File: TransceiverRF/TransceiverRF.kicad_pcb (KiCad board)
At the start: 2 copper layers, 48 parts, among them U1 CC1101, U2 CON_SMA, U3 CC2500, U4 CON_SMA, Y1 26 MHz, Y2 26 MHz

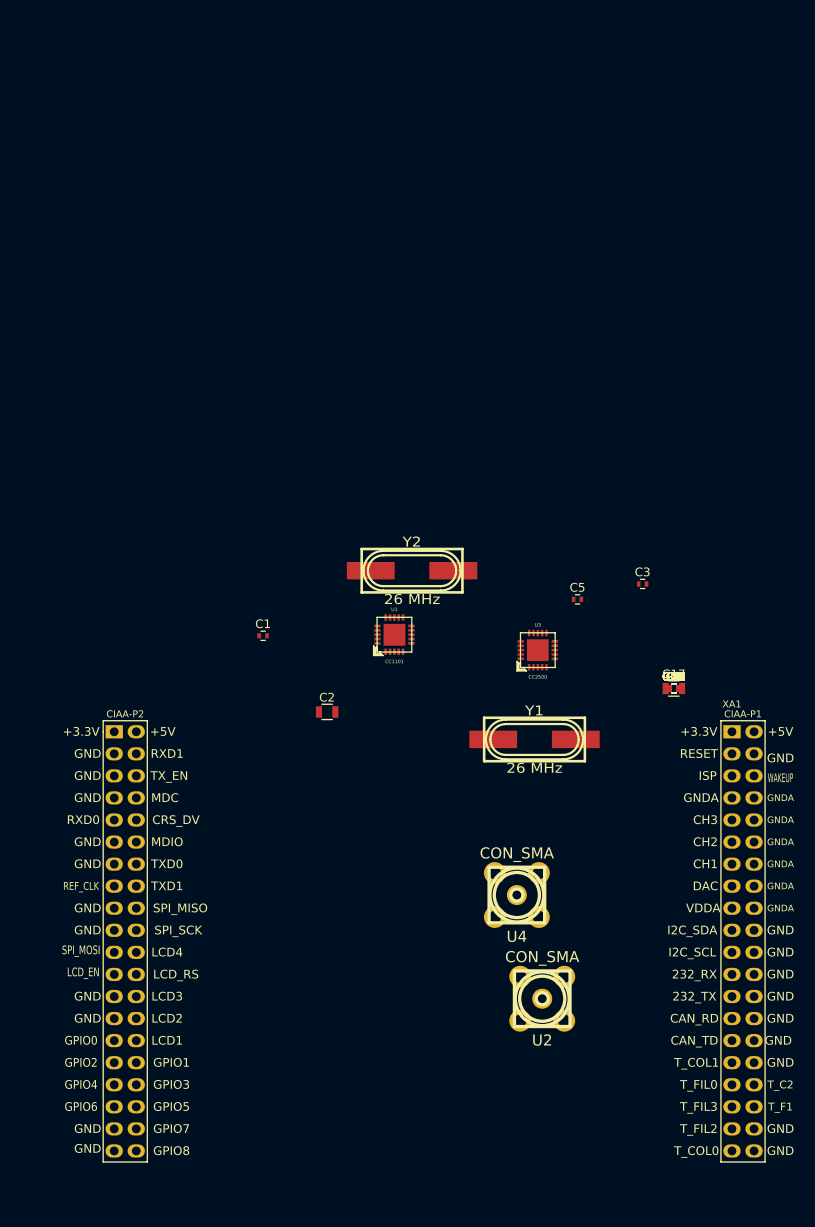
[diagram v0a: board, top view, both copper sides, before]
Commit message: agrego pcb
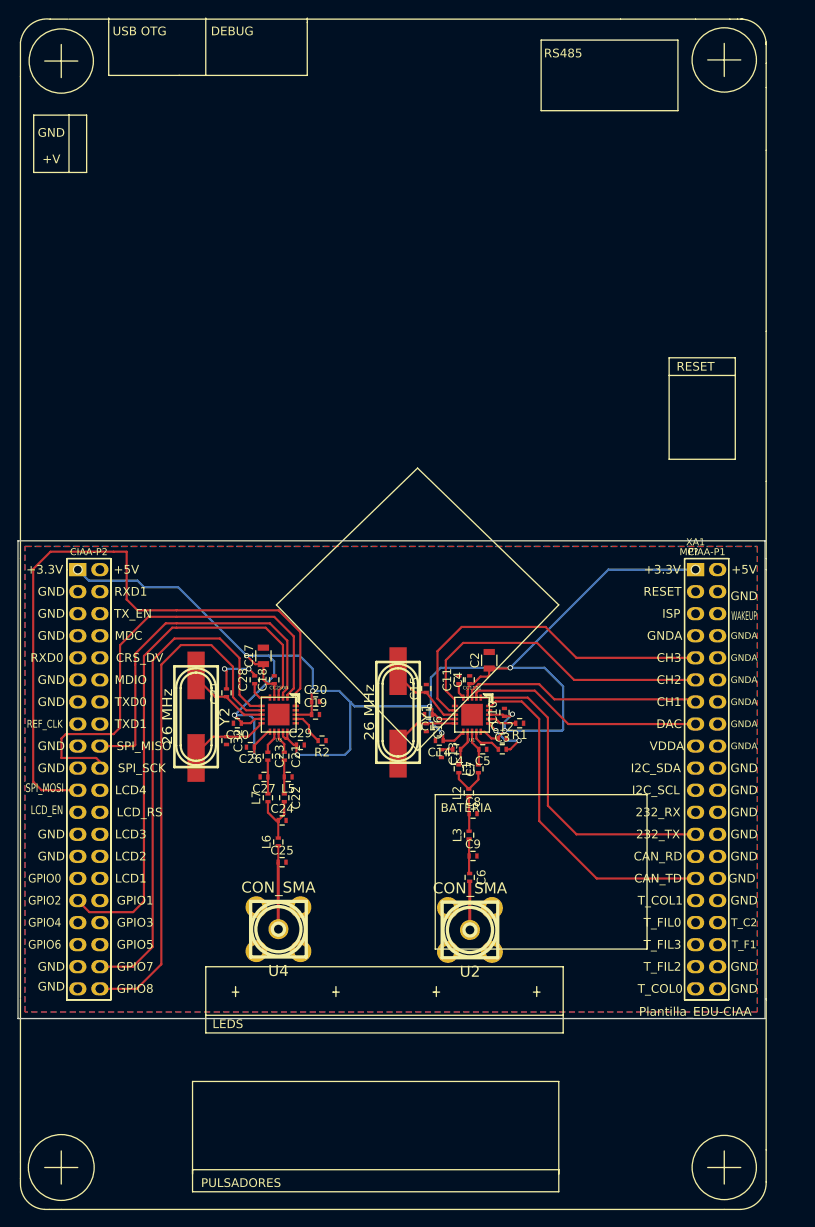
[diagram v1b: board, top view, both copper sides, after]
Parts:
- added MP?: Plantilla_EDU-CIAA, TransceiverRF:Plantilla_EDU-CIAA, F.Cu at (151.0, 91.3)
- moved C32 51.8 mm to (97.0, 111.0), turned to 270 degrees
- moved C31 51.5 mm to (97.0, 105.5), turned to 90 degrees
- moved C30 50.4 mm to (98.2, 109.0), turned to 180 degrees
- moved C25 49.3 mm to (103.4, 125.0)
- moved C26 49.2 mm to (99.8, 111.8), turned to 180 degrees
- moved L6 48.8 mm to (103.0, 122.7), turned to 90 degrees
- moved L7 48.4 mm to (101.8, 117.6), turned to 90 degrees
- moved C27 48.3 mm to (101.3, 115.2), turned to 180 degrees
- moved C28 48.3 mm to (100.2, 104.0), turned to 90 degrees
- moved C24 47.6 mm to (103.4, 120.2)
- moved C17 47.4 mm to (101.2, 101.2), turned to 90 degrees
- moved C23 47.4 mm to (101.8, 112.8), turned to 270 degrees
- moved C22 46.6 mm to (103.7, 117.6), turned to 270 degrees
- moved C18 46.0 mm to (102.5, 104.0), turned to 90 degrees
- moved L5 45.6 mm to (104.1, 115.2), turned to 180 degrees
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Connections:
- C1 pad 2: Net-(C1-Pad2) -> Earth
- C10 pad 2: Net-(C10-Pad2) -> Earth
- C11 pad 2: Net-(C11-Pad2) -> Earth
- C12 pad 2: Net-(C12-Pad2) -> Earth
- C13 pad 2: Net-(C13-Pad2) -> Earth
- C14 pad 2: Net-(C14-Pad2) -> Earth
- C15 pad 2: Net-(C15-Pad2) -> Earth
- C16 pad 2: Net-(C16-Pad2) -> Earth
- C17 pad 2: Net-(C17-Pad2) -> Earth
- C18 pad 2: Net-(C18-Pad2) -> Earth
- C19 pad 2: Net-(C19-Pad2) -> Earth
- C2 pad 2: Net-(C2-Pad2) -> Earth
- C20 pad 2: Net-(C20-Pad2) -> Earth
- C24 pad 2: Net-(C24-Pad2) -> Earth
- C25 pad 2: Net-(C25-Pad2) -> Earth
- C26 pad 2: Net-(C26-Pad2) -> Earth
- C27 pad 2: Net-(C27-Pad2) -> Earth
- C28 pad 2: Net-(C28-Pad2) -> Earth
- C29 pad 2: Net-(C29-Pad2) -> Earth
- C3 pad 2: Net-(C3-Pad2) -> Earth
- C30 pad 2: Net-(C30-Pad2) -> Earth
- C31 pad 2: Net-(C31-Pad2) -> Earth
- C32 pad 2: Net-(C32-Pad2) -> Earth
- C4 pad 2: Net-(C4-Pad2) -> Earth
- C5 pad 1: Net-(C5-Pad1) -> Earth
- C8 pad 2: Net-(C8-Pad2) -> Earth
- C9 pad 2: Net-(C9-Pad2) -> Earth
- L5 pad 1: Net-(L5-Pad1) -> Earth
- R1 pad 1: Net-(R1-Pad1) -> Earth
- R2 pad 1: Net-(R2-Pad1) -> Earth
- U1 pad 16: Net-(U1-Pad16) -> Earth
- U1 pad 19: Net-(U1-Pad19) -> Earth
- U1 pad 3: /Conectores/GDO1(opcional)_CC1101 -> /CC1101/GDO2(opcional)_CC1101
- U2 pad 2: Net-(U2-Pad2) -> Earth
- U3 pad 16: Net-(U3-Pad16) -> Earth
- U3 pad 19: Net-(U3-Pad19) -> Earth
- U4 pad 2: Net-(U4-Pad2) -> Earth
- XA1 pad 11: Net-(XA1-Pad11) -> /CC1101/GDO1(opcional)_CC1101
- XA1 pad 13: Net-(XA1-Pad13) -> /CC1101/GDO2(opcional)_CC1101
- XA1 pad 15: Net-(XA1-Pad15) -> /CC1101/SO_CC1101
- XA1 pad 20: Net-(XA1-Pad20) -> Earth
- XA1 pad 22: Net-(XA1-Pad20) -> Earth
- XA1 pad 24: Net-(XA1-Pad20) -> Earth
- XA1 pad 25: Net-(XA1-Pad25) -> /Conectores/SCLK_1101
- XA1 pad 26: Net-(XA1-Pad20) -> Earth
- XA1 pad 28: Net-(XA1-Pad20) -> Earth
- XA1 pad 29: Net-(XA1-Pad29) -> /CC1101/SI_CC1101
- XA1 pad 30: Net-(XA1-Pad20) -> Earth
- XA1 pad 32: Net-(XA1-Pad20) -> Earth
- XA1 pad 38: Net-(XA1-Pad20) -> Earth
- XA1 pad 4: Net-(XA1-Pad20) -> Earth
- XA1 pad 40: Net-(XA1-Pad20) -> Earth
- XA1 pad 43: Net-(XA1-Pad43) -> Earth
- XA1 pad 44: /CC1101/SO_CC1101 -> Net-(XA1-Pad44)
- XA1 pad 45: Net-(XA1-Pad43) -> Earth
- XA1 pad 46: /CC1101/SI_CC1101 -> Net-(XA1-Pad46)
- XA1 pad 47: Net-(XA1-Pad43) -> Earth
- XA1 pad 51: Net-(XA1-Pad43) -> Earth
- XA1 pad 53: Net-(XA1-Pad43) -> Earth
- XA1 pad 55: /Conectores/SCLK_1101 -> Net-(XA1-Pad55)
- XA1 pad 57: Net-(XA1-Pad43) -> Earth
- XA1 pad 59: Net-(XA1-Pad43) -> Earth
- XA1 pad 65: Net-(XA1-Pad43) -> Earth
- XA1 pad 67: Net-(XA1-Pad43) -> Earth
- XA1 pad 69: /CC2500/GDO1(opcional)_CC2500 -> Net-(XA1-Pad69)
- XA1 pad 72: /Conectores/GDO1(opcional)_CC1101 -> Net-(XA1-Pad72)
- XA1 pad 73: /CC2500/CSn_CC2500 -> Net-(XA1-Pad73)
- XA1 pad 74: /CC1101/GDO1(opcional)_CC1101 -> Net-(XA1-Pad74)
- XA1 pad 76: /CC1101/CSn_CC1101 -> Net-(XA1-Pad76)
- XA1 pad 77: Net-(XA1-Pad43) -> Earth
- XA1 pad 78: Net-(XA1-Pad78) -> /CC2500/GDO1(opcional)_CC2500
- XA1 pad 79: Net-(XA1-Pad43) -> Earth
- XA1 pad 80: Net-(XA1-Pad80) -> /CC2500/CSn_CC2500
- XA1 pad 9: Net-(XA1-Pad9) -> /CC1101/CSn_CC1101
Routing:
- net +3V3: track 0.00 -> 188.7 mm, vias 0 -> 10
- net /CC2500/SI_CC2500: track 0.00 -> 77.4 mm
- net /CC2500/GDO2(opcional)_CC2500: track 0.00 -> 61.4 mm
- net /CC2500/CSn_CC2500: track 0.00 -> 60.4 mm
- net /CC2500/GDO1(opcional)_CC2500: track 0.00 -> 59.3 mm
- net /Conectores/SCLK_2500: track 0.00 -> 54.0 mm
- net /CC2500/SO_CC2500: track 0.00 -> 41.2 mm
- net /CC1101/CSn_CC1101: track 0.00 -> 40.4 mm
- net /CC1101/SI_CC1101: track 0.00 -> 39.3 mm
- net /Conectores/SCLK_1101: track 0.00 -> 37.2 mm
- net /CC1101/GDO1(opcional)_CC1101: track 0.00 -> 37.1 mm
- net /CC1101/GDO2(opcional)_CC1101: track 0.00 -> 27.7 mm
- net /CC1101/SO_CC1101: track 0.00 -> 27.5 mm
- net Earth: track 0.00 -> 12.5 mm, vias 0 -> 4
- net Net-(C16-Pad1): track 0.00 -> 10.5 mm
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- added copper zone on B.Cu, net Earth
- added copper zone on F.Cu, net Earth
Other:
- board outline added: 86 x 55 mm
- net class Default: clearance 0.2 -> 0.12
- rule trace_clearance: 0.2 -> 0.12
